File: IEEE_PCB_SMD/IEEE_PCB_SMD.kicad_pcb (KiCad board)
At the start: 2 copper layers, 98.9 x 105.3 mm, 18 parts, among them U1 555, U2 4017, U3 EG1218, U4 1058TR

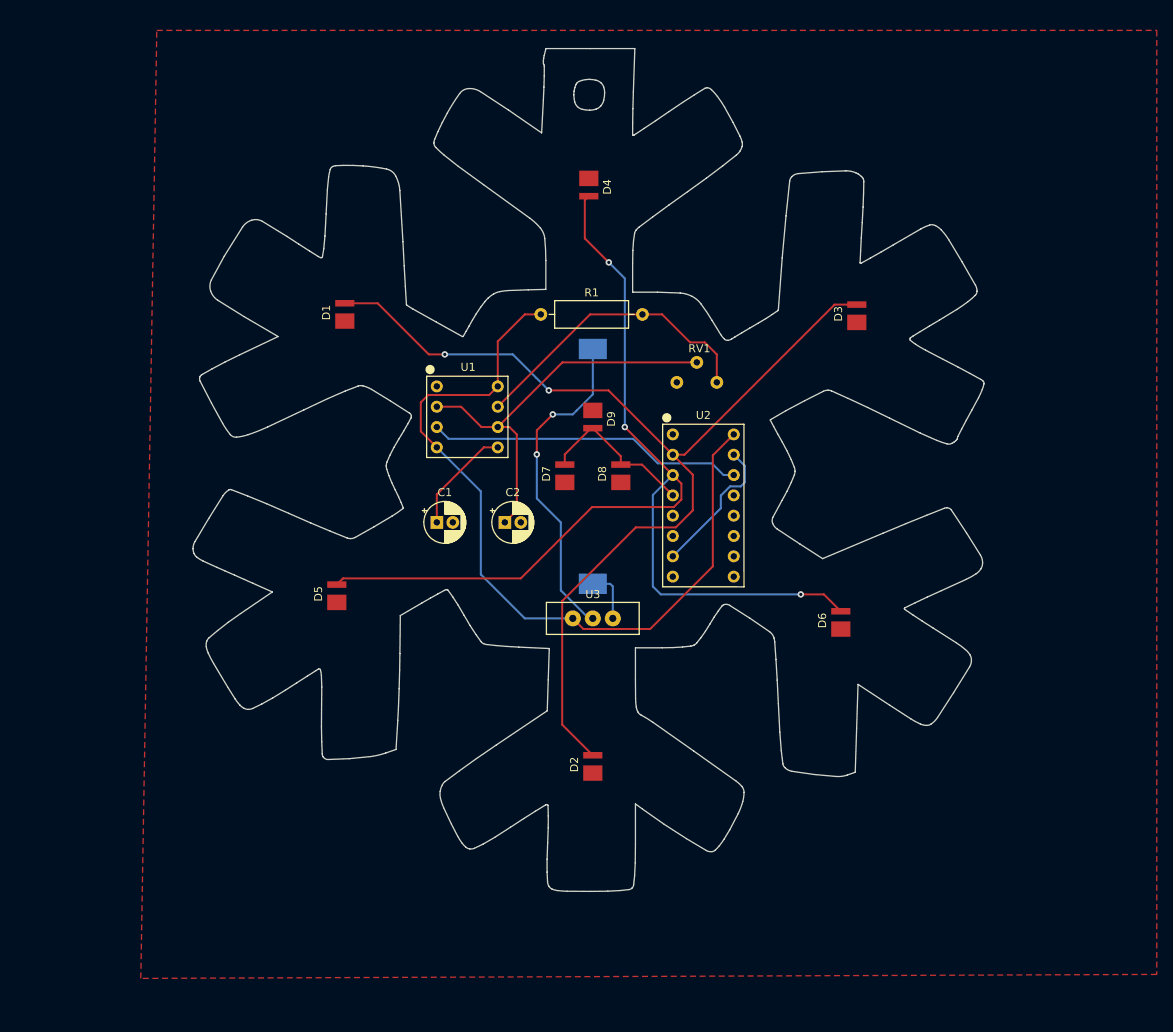
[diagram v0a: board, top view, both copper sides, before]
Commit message: SMD Rev3
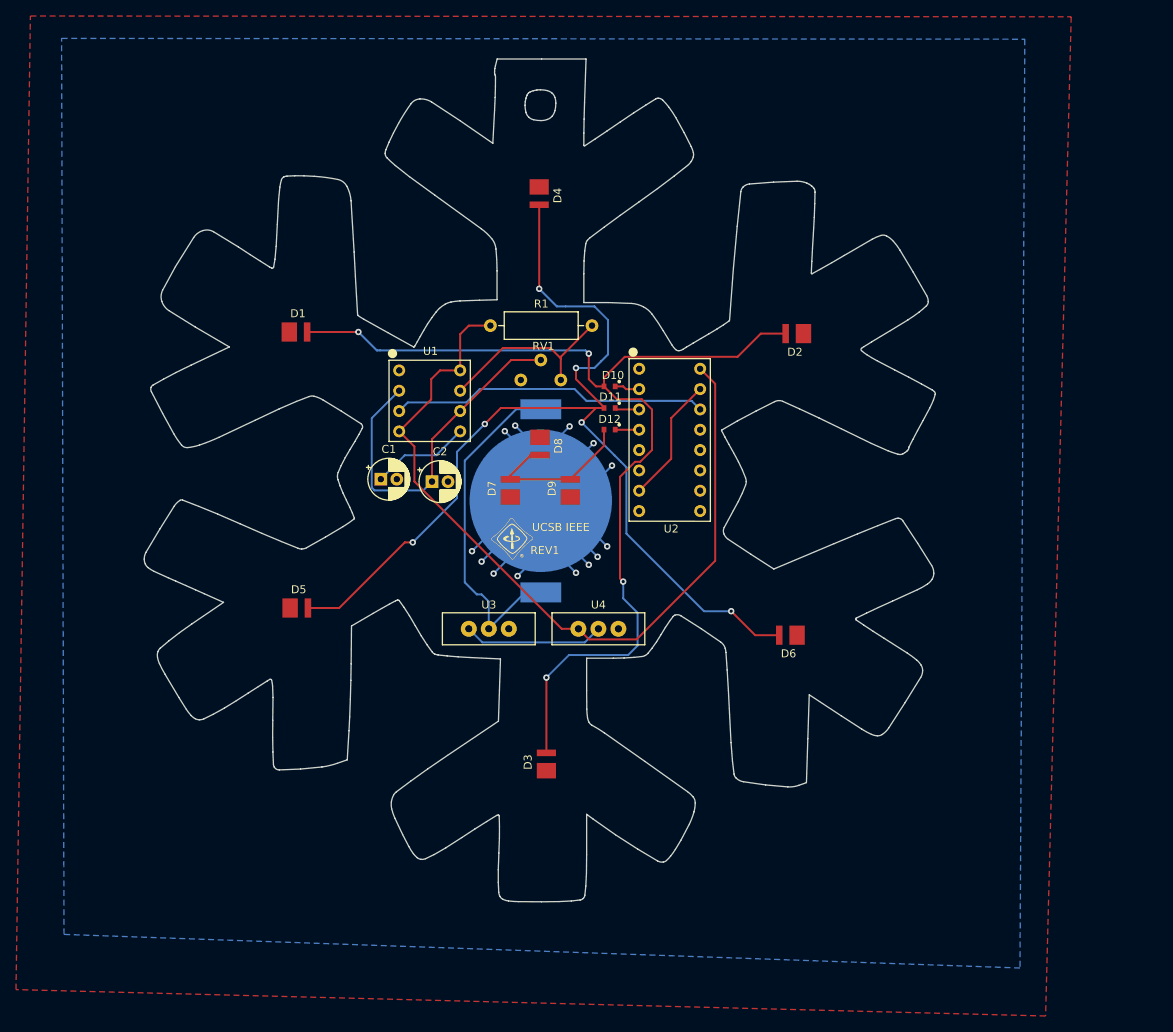
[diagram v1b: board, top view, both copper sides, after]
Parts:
- added D10: D, IEEE_PCB_Ornament:SDM20U40Q, F.Cu at (153.6, 81.5)
- added D11: D, IEEE_PCB_Ornament:SDM20U40Q, F.Cu at (153.6, 84.2)
- added D12: D, IEEE_PCB_Ornament:SDM20U40Q, F.Cu at (153.6, 86.9)
- added G***: LOGO, Logos:IEEE Logo, F.Cu at (141.4, 100.6)
- added U5: CR2025TR, IEEE_PCB_Ornament:CR2025TR, F.Cu at (145.0, 95.8)
- RV1: value 500K -> 100K
- U4: value 1058TR -> EG1218; footprint IEEE_PCB_Ornament:1058TR -> IEEE_PCB_Ornament:EG1218
- moved D3 68.2 mm to (145.7, 128.7)
- moved D2 59.8 mm to (177.0, 74.9), turned to 90 degrees
- moved U4 20.3 mm to (152.2, 111.8), turned to 0 degrees
- moved RV1 19.5 mm to (145.0, 80.7)
- moved U3 13.1 mm to (138.5, 111.8)
- moved D8 10.9 mm to (144.9, 88.7), turned to 180 degrees
- moved C2 10.4 mm to (131.4, 93.4)
- moved D9 9.58 mm to (148.7, 94.5), turned to 0 degrees
- moved U2 9.21 mm to (157.3, 79.3)
- moved C1 8.84 mm to (125.0, 93.1)
- moved D7 7.04 mm to (141.2, 94.5)
- moved D6 6.50 mm to (176.2, 112.6), turned to 90 degrees
- moved D1 6.48 mm to (114.4, 74.7), turned to 270 degrees
- moved R1 6.45 mm to (138.7, 73.9)
- moved D4 6.29 mm to (144.8, 57.4)
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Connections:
- D1 pad 2: Net-(D1-Pad2) -> ALLON
- D2 pad 2: Net-(D1-Pad2) -> ALLON
- D3 pad 2: Net-(D1-Pad2) -> ALLON
- D4 pad 2: Net-(D4-Pad2) -> ALLON
- D5 pad 2: Net-(D4-Pad2) -> ALLON
- D6 pad 2: Net-(D4-Pad2) -> ALLON
- D7 pad 2: Net-(D7-Pad2) -> ALLON
- D8 pad 2: Net-(D7-Pad2) -> ALLON
- D9 pad 2: Net-(D7-Pad2) -> ALLON
- U2 pad 2: Net-(D1-Pad2) -> Net-(D10-Pad2)
- U2 pad 3: Net-(D4-Pad2) -> Net-(D11-Pad2)
- U2 pad 4: Net-(D7-Pad2) -> Net-(D12-Pad2)
- U3 pad 1: +3V3 -> Net-(U3-Pad1)
- U3 pad 3: GND -> Net-(U3-Pad3)
- U4 pad 1: Net-(U3-Pad2) -> +3V3
- U4 pad 2: GND -> Net-(U3-Pad1)
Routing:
- net ALLON: track 0.00 -> 283.9 mm, vias 0 -> 10
- net GND: track 6.63 -> 148.7 mm, vias 0 -> 13
- net Net-(D4-Pad2): track 130.3 -> 0.00 mm, vias 3 -> 0
- net Net-(D1-Pad2): track 129.5 -> 0.00 mm, vias 2 -> 0
- net Net-(D7-Pad2): track 20.2 -> 0.00 mm
- net Net-(U3-Pad1): track 0.00 -> 17.6 mm
- net Net-(R1-Pad2): track 38.1 -> 23.7 mm
- net Net-(C2-Pad1): track 51.3 -> 44.7 mm
- net Net-(D10-Pad2): track 0.00 -> 3.14 mm
- net Net-(D11-Pad2): track 0.00 -> 3.07 mm
- net Net-(D12-Pad2): track 0.00 -> 3.01 mm
- net +3V3: track 100.1 -> 102.7 mm
- net Net-(U2-Pad15): track 17.8 -> 15.9 mm
- net Net-(U3-Pad2): track 41.2 -> 43.2 mm, vias 2 -> 0
- net Net-(C1-Pad1): track 13.6 -> 12.4 mm
- added copper zone on B.Cu, net ALLON
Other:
- board size 98.9 x 105.3 mm -> 98.9 x 105.4 mm
- board text added: "REV1"
- board text added: "UCSB IEEE"
